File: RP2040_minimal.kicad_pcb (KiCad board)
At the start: 2 copper layers, 52 x 51 mm, 34 parts, among them J1 USB_B_Micro, J2 Conn_01x02, J3 Conn_02x18_Odd_Even, J4 Conn_02x18_Odd_Even, U1 NCP1117-3.3_SOT223, U2 W25Q128JVS, U3 RP2040, Y1 ABLS-12.000MHZ-B4-T

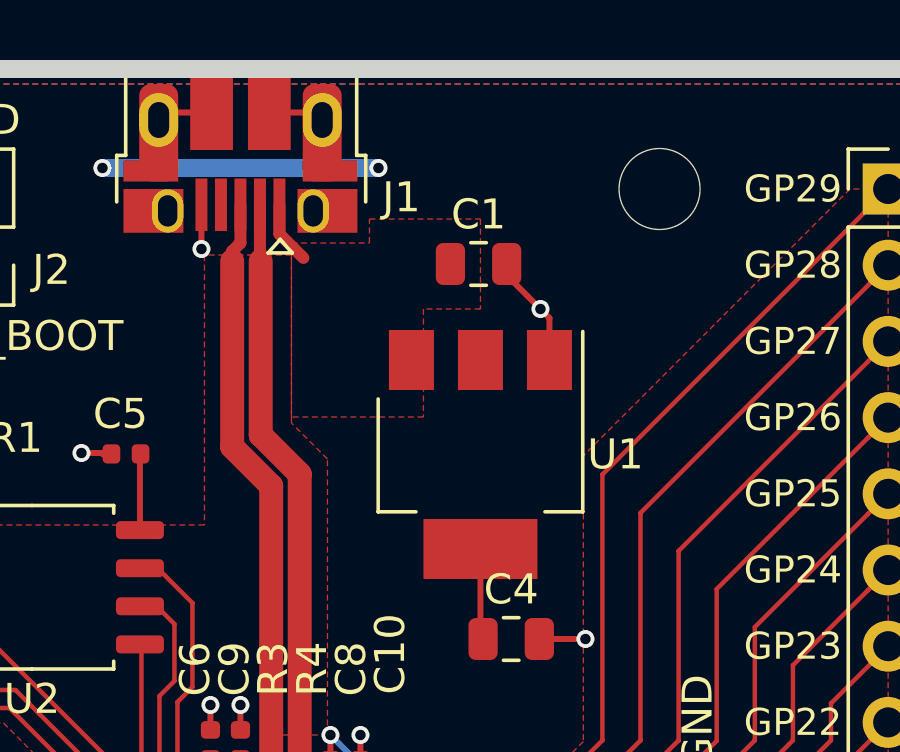
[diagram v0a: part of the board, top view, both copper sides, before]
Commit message: A random move
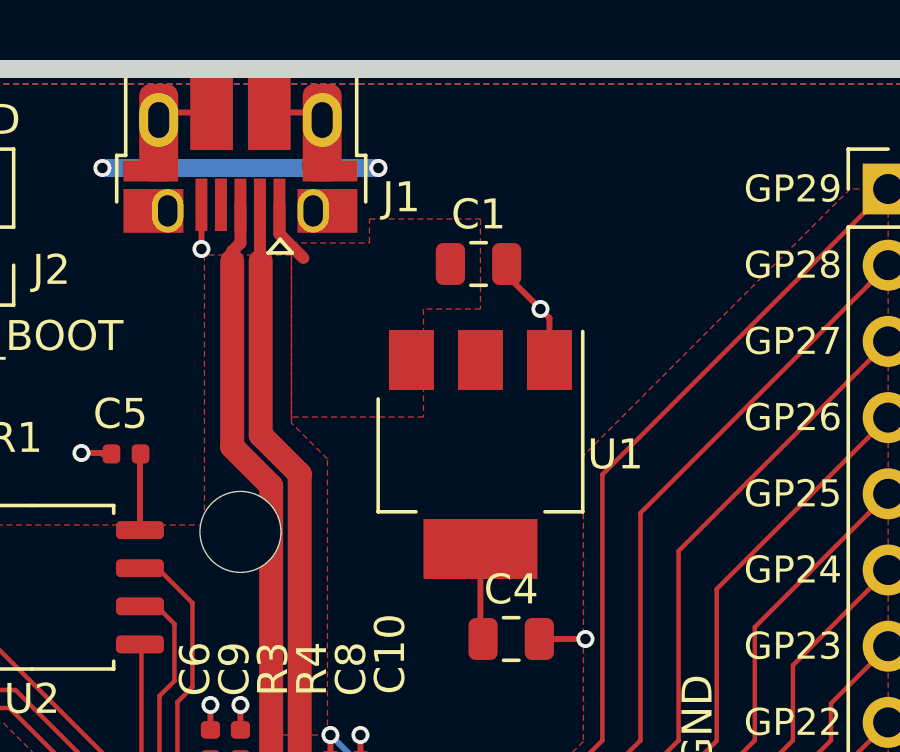
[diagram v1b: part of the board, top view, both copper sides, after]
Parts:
- moved H2 18.1 mm to (100.0, 85.4)
